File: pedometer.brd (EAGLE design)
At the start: 160 x 100 mm, 2 parts, among them U1 LSM6DSO32TRLGA-14L_2P5X3X0P83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

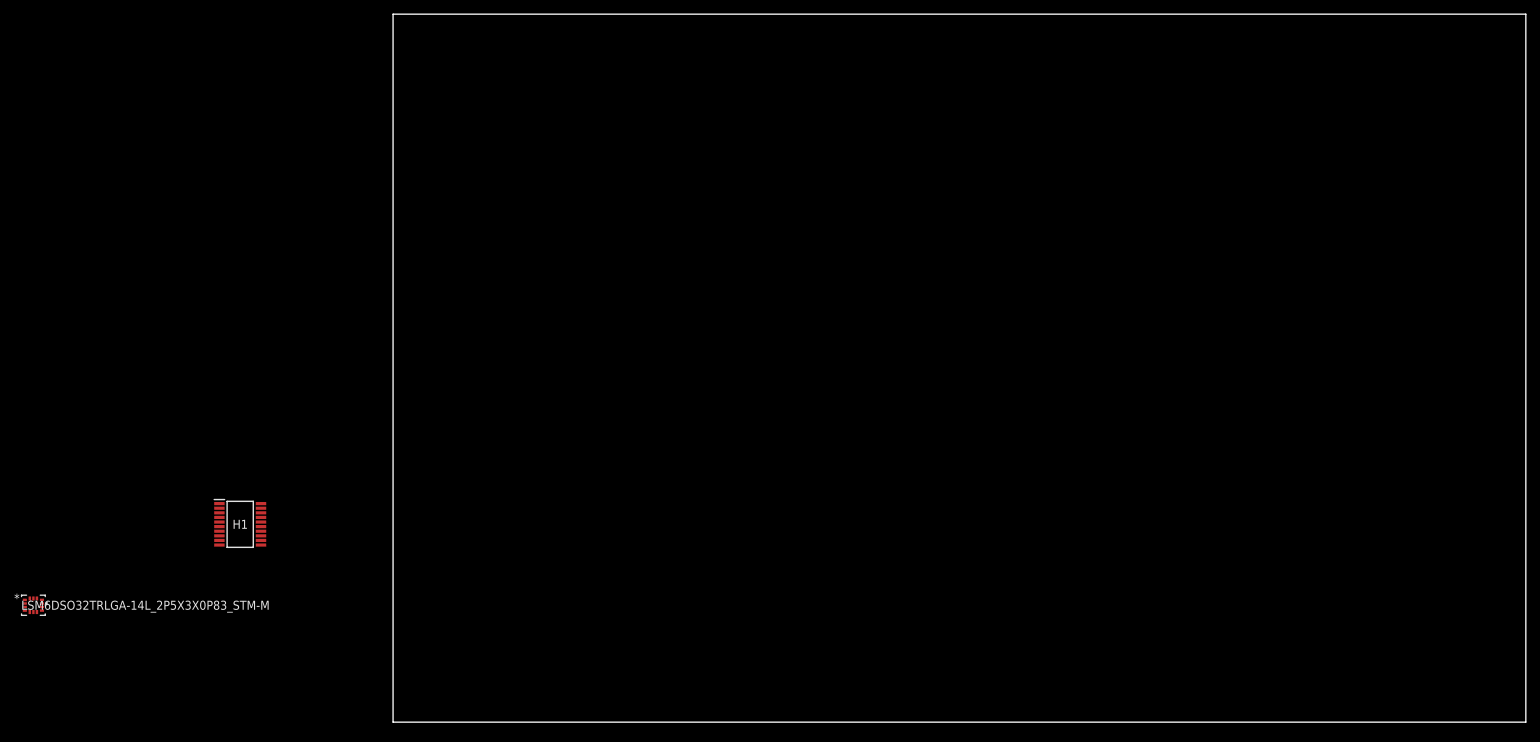
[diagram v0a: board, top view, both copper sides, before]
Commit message: COmpleted board files
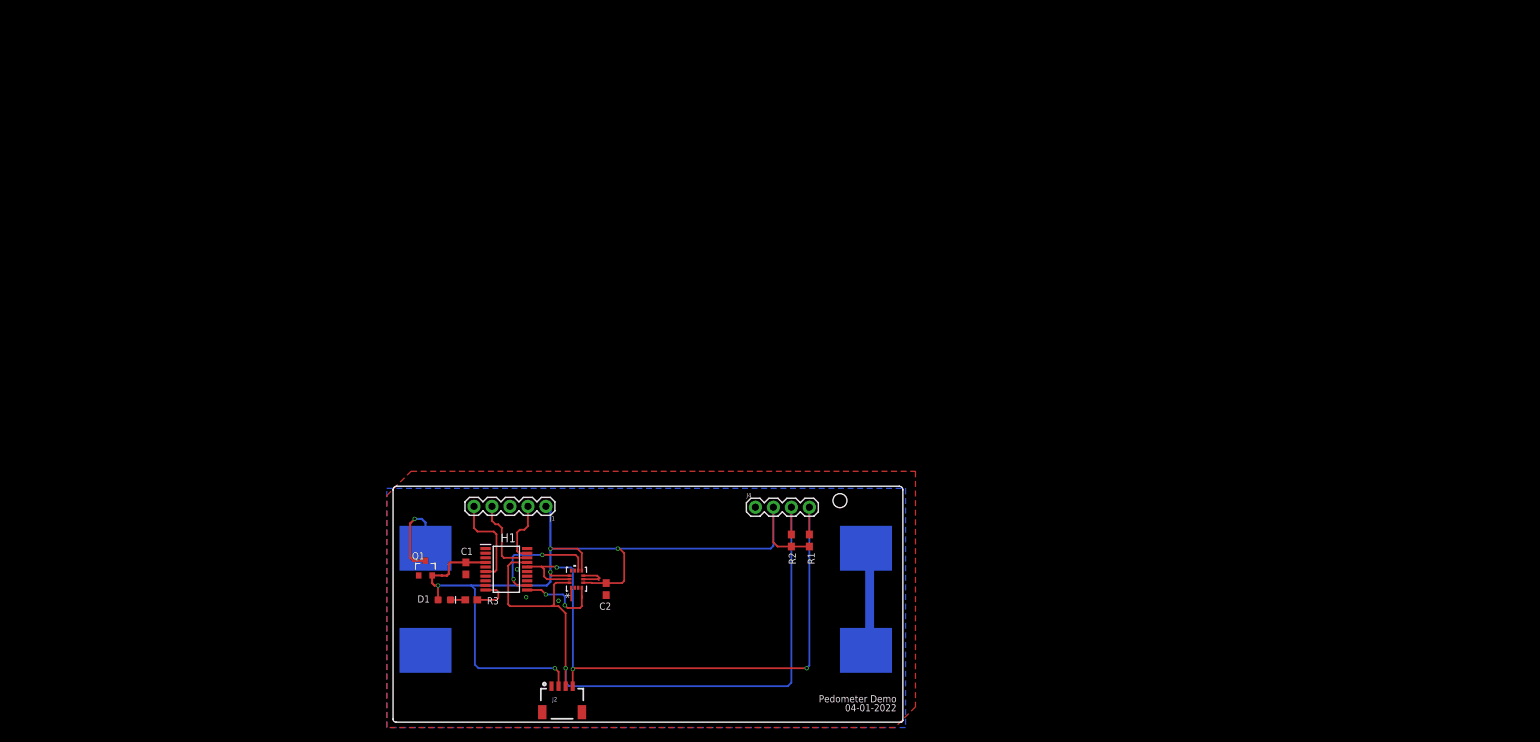
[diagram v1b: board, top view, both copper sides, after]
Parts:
- added C1, C2: 0.1uF, SparkFun-Capacitors:0603
- added D1: BLUE, SparkFun-LED:LED-0603
- added J1: (no value), SparkFun-Connectors:1X05
- added J2: (no value), SparkFun-Connectors:1X04_1MM_RA
- added J3: 1012, 1012:1012
- added J4: (no value), SparkFun-Connectors:1X04
- added Q1: 2.5A/30V/105mΩ, SparkFun-DiscreteSemi:SOT23-3
- added R1, R2: 2.2k, SparkFun-Resistors:0603
- added R3: 220, SparkFun-Resistors:0603
- moved U1 76.8 mm to (25.9, 20.2), turned to 90 degrees
- moved H1 38.1 mm to (16.0, 21.6)
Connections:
- removed net VDD/VDDA: H1.4
- removed net VDDIO: U1.5
- removed net VSS/VSSA: H1.5
- new net GND: C1.1, C2.1, H1.5, J1.3, J2.1, J3.3, J4.1, Q1.1, U1.1, U1.6, U1.7
- new net INT1: H1.11, U1.4
- new net INT2: H1.12, U1.9
- new net N$1: J3.1, J3.2
- new net N$2: J3.4, Q1.3
- new net N$3: H1.10, R3.1
- new net N$4: D1.C, R3.2
- new net NRST: H1.6, J1.5
- new net SCL: H1.16, J2.4, J4.4, R1.1, U1.13
- new net SDA: H1.17, J2.3, J4.3, R2.1, U1.14
- new net SWCLK: H1.19, J1.2
- new net SWDIO: H1.18, J1.4
- net VDD: now also C1.2, C2.2, D1.A, H1.4, J1.1, J2.2, J4.2, Q1.2, R1.2, R2.2, U1.12, U1.5
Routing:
- net VDD: track 0.00 -> 134.6 mm, vias 0 -> 5
- net SDA: track 0.00 -> 95.7 mm, vias 0 -> 1
- net SCL: track 0.00 -> 88.3 mm, vias 0 -> 3
- net INT2: track 0.00 -> 17.1 mm, vias 0 -> 2
- net N$1: track 0.00 -> 15.1 mm
- net N$2: track 0.00 -> 13.4 mm, vias 0 -> 1
- net NRST: track 0.00 -> 13.3 mm
- net INT1: track 0.00 -> 12.2 mm, vias 0 -> 2
- net SWDIO: track 0.00 -> 11.5 mm
- net SWCLK: track 0.00 -> 8.88 mm
- net GND: track 0.00 -> 6.60 mm, vias 0 -> 3
- net N$3: track 0.00 -> 5.86 mm
- net N$4: track 0.00 -> 2.08 mm
- added copper zone on layer 1, net GND
- added copper zone on layer 16, net GND
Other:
- board size 160 x 100 mm -> 72 x 33.3 mm
- board text added: "+"
- board text added: "-"
- board text added: "04-01-2022"
- board text added: "Pedometer Demo"
